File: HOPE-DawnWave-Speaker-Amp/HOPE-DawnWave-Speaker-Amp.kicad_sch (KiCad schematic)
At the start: 9 parts, among them J1 Screw_Terminal_01x02, U1 MAX98357A

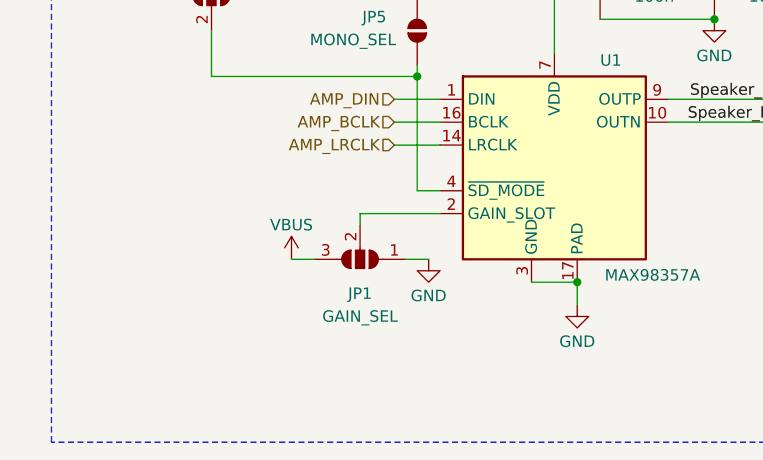
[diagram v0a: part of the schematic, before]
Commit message: fab files generated, pcb finalized
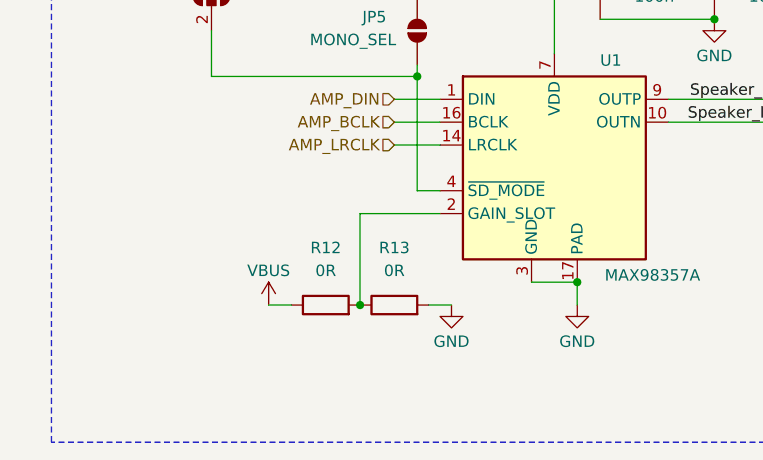
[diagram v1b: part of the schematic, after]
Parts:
- removed JP1: GAIN_SEL, Jumper:SolderJumper-3_P2.0mm_Open_TrianglePad1.0x1.5mm, symbol Jumper:SolderJumper_3_Open
- added R12, R13: 0R, Resistor_SMD:R_0402_1005Metric_Pad0.72x0.64mm_HandSolder, symbol Device:R
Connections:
- net GND: now also R13.2
- net VBUS: now also R12.1
- net at U1.2 (GAIN_SLOT): now also R12.2, R13.1
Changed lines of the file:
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@@
+	)
+	(junction
+		(at 119.38 116.84)
+		(diameter 0)
+		(color 0 0 0 0)
 	)
 	(junction
@@
 	(wire
 		(pts
-			(xy 124.46 111.76) (xy 127 111.76)
+			(xy 127 116.84) (xy 129.54 116.84)
 		)
 		(stroke
@@
 	(wire
 		(pts
-			(xy 111.76 111.76) (xy 114.3 111.76)
-		)
-		(stroke
-			(width 0)
-			(type default)
-		)
-	)
-	(wire
-		(pts
-			(xy 119.38 106.68) (xy 119.38 107.95)
+			(xy 109.22 116.84) (xy 111.76 116.84)
+		)
+		(stroke
+			(width 0)
+			(type default)
+		)
+	)
+	(wire
+		(pts
+			(xy 119.38 106.68) (xy 119.38 116.84)
 		)
 		(stroke
@@
 	(symbol
 		(lib_id "power:VBUS")
-		(at 111.76 111.76 0)
+		(at 109.22 116.84 0)
 		(unit 1)
 		(exclude_from_sim no)
@@
 		(dnp no)
 		(property "Reference" "#PWR02"
-			(at 111.76 115.57 0)
+			(at 109.22 120.65 0)
 			(effects
 				(font
@@
 		)
 		(property "Value" "VBUS"
-			(at 111.76 107.95 0)
+			(at 109.22 113.03 0)
 			(effects
 				(font
@@
 		)
 		(property "Footprint" ""
-			(at 111.76 111.76 0)
+			(at 109.22 116.84 0)
 			(effects
 				(font
@@
 		)
 		(property "Datasheet" ""
-			(at 111.76 111.76 0)
+			(at 109.22 116.84 0)
 			(effects
 				(font
@@
 		)
 		(property "Description" "Power symbol creates a global label with name \"VBUS\""
-			(at 111.76 111.76 0)
+			(at 109.22 116.84 0)
 			(effects
 				(font
@@
 	(symbol
 		(lib_id "power:GND")
-		(at 127 111.76 0)
+		(at 129.54 116.84 0)
 		(unit 1)
 		(exclude_from_sim no)
@@
 		(dnp no)
 		(property "Reference" "#PWR04"
-			(at 127 118.11 0)
+			(at 129.54 123.19 0)
 			(effects
 				(font
@@
 		)
 		(property "Value" "GND"
-			(at 127 115.824 0)
+			(at 129.54 120.904 0)
 			(effects
 				(font
@@
 		)
 		(property "Footprint" ""
-			(at 127 111.76 0)
+			(at 129.54 116.84 0)
 			(effects
 				(font
@@
 		)
 		(property "Datasheet" ""
-			(at 127 111.76 0)
+			(at 129.54 116.84 0)
 			(effects
 				(font
@@
 		)
 		(property "Description" "Power symbol creates a global label with name \"GND\" , ground"
-			(at 127 111.76 0)
+			(at 129.54 116.84 0)
 			(effects
 				(font
@@
 	)
 	(symbol
+		(lib_id "Device:R")
+		(at 115.57 116.84 90)
+		(unit 1)
+		(exclude_from_sim no)
+		(in_bom yes)
+		(on_board yes)
+		(dnp no)
+		(fields_autoplaced yes)
+		(property "Reference" "R12"
+			(at 115.57 110.49 90)
+			(effects
+				(font
+					(size 1.27 1.27)
+				)
+			)
+		)
+		(property "Value" "0R"
+			(at 115.57 113.03 90)
+			(effects
+				(font
+					(size 1.27 1.27)
+				)
+			)
+		)
+		(property "Footprint" "Resistor_SMD:R_0402_1005Metric_Pad0.72x0.64mm_HandSolder"
+			(at 115.57 118.618 90)
+			(effects
+				(font
+					(size 1.27 1.27)
+				)
+				(hide yes)
+			)
+		)
+		(property "Datasheet" "~"
+			(at 115.57 116.84 0)
+			(effects
+				(font
+					(size 1.27 1.27)
+				)
+				(hide yes)
+			)
+		)
+		(property "Description" "Resistor"
+			(at 115.57 116.84 0)
+			(effects
+				(font
+					(size 1.27 1.27)
+				)
+				(hide yes)
+			)
+		)
+		(pin "1"
+		)
+		(pin "2"
+		)
+		(instances
+			(project ""
+				(path "/b8bc6909-42e2-441d-8c23-4bce71b0ba4f/01173765-a7e8-4b6a-9749-4cb153e0b2d3"
+					(reference "R12")
+					(unit 1)
+				)
+			)
+		)
+	)
+	(symbol
+		(lib_id "Device:R")
+		(at 123.19 116.84 90)
+		(unit 1)
+		(exclude_from_sim no)
+		(in_bom yes)
+		(on_board yes)
+		(dnp no)
+		(fields_autoplaced yes)
+		(property "Reference" "R13"
+			(at 123.19 110.49 90)
+			(effects
+				(font
+					(size 1.27 1.27)
+				)
+			)
+		)
+		(property "Value" "0R"
+			(at 123.19 113.03 90)
+			(effects
+				(font
+					(size 1.27 1.27)
+				)
+			)
+		)
+		(property "Footprint" "Resistor_SMD:R_0402_1005Metric_Pad0.72x0.64mm_HandSolder"
+			(at 123.19 118.618 90)
+			(effects
+				(font
+					(size 1.27 1.27)
+				)
+				(hide yes)
+			)
+		)
+		(property "Datasheet" "~"
+			(at 123.19 116.84 0)
+			(effects
+				(font
+					(size 1.27 1.27)
+				)
+				(hide yes)
+			)
+		)
+		(property "Description" "Resistor"
+			(at 123.19 116.84 0)
+			(effects
+				(font
+					(size 1.27 1.27)
+				)
+				(hide yes)
+			)
+		)
+		(pin "1"
+		)
+		(pin "2"
+		)
+		(instances
+			(project ""
+				(path "/b8bc6909-42e2-441d-8c23-4bce71b0ba4f/01173765-a7e8-4b6a-9749-4cb153e0b2d3"
+					(reference "R13")
+					(unit 1)
+				)
+			)
+		)
+	)
+	(symbol
 		(lib_id "power:+3.3V")
 		(at 95.25 74.93 0)
@@
 					(unit 1)
 				)
-			)
-		)
-	)
-	(symbol
-		(lib_id "Jumper:SolderJumper_3_Open")
-		(at 119.38 111.76 180)
-		(unit 1)
-		(exclude_from_sim yes)
-		(in_bom no)
-		(on_board yes)
-		(dnp no)
-		(fields_autoplaced yes)
-		(property "Reference" "JP1"
-			(at 119.38 115.57 0)
-			(effects
-				(font
-					(size 1.27 1.27)
-				)
-			)
-		)
-		(property "Value" "GAIN_SEL"
-			(at 119.38 118.11 0)
-			(effects
-				(font
-					(size 1.27 1.27)
-				)
-			)
-		)
-		(property "Footprint" "Jumper:SolderJumper-3_P2.0mm_Open_TrianglePad1.0x1.5mm"
-			(at 119.38 111.76 0)
-			(effects
-				(font
-					(size 1.27 1.27)
-				)
-				(hide yes)
-			)
-		)
-		(property "Datasheet" "~"
-			(at 119.38 111.76 0)
-			(effects
-				(font
-					(size 1.27 1.27)
-				)
-				(hide yes)
-			)
-		)
-		(property "Description" "Solder Jumper, 3-pole, open"
-			(at 119.38 111.76 0)
-			(effects
-				(font
-					(size 1.27 1.27)
-				)
-				(hide yes)
-			)
-		)
-		(pin "1"
-		)
-		(pin "3"
-		)
-		(pin "2"
-		)
-		(instances
-			(project "HOPE-DawnWave-Speaker-Amp"
-				(path "/9b63a486-35b2-4834-a35d-68d229baf124"
-					(reference "JP1")
-					(unit 1)
-				)
-			)
-			(project "HOPE-DawnWave-Speaker-Amp"
-				(path "/b8bc6909-42e2-441d-8c23-4bce71b0ba4f/01173765-a7e8-4b6a-9749-4cb153e0b2d3"
-					(reference "JP4")
-					(unit 1)
-				)
